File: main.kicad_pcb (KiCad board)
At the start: 2 copper layers, 82.8 x 33.2 mm, 34 parts, among them J1 USB_C_Receptacle_USB2.0_14P, SW1 SW_PUSH, SW2 SW_PUSH, SW3 SW_PUSH, SW4 SW_PUSH, SW5 SW_PUSH, U1 NCP1117-3.3_SOT223, U2 RP2040, U3 W25Q128JVS, Y1 ABM8-272-T3

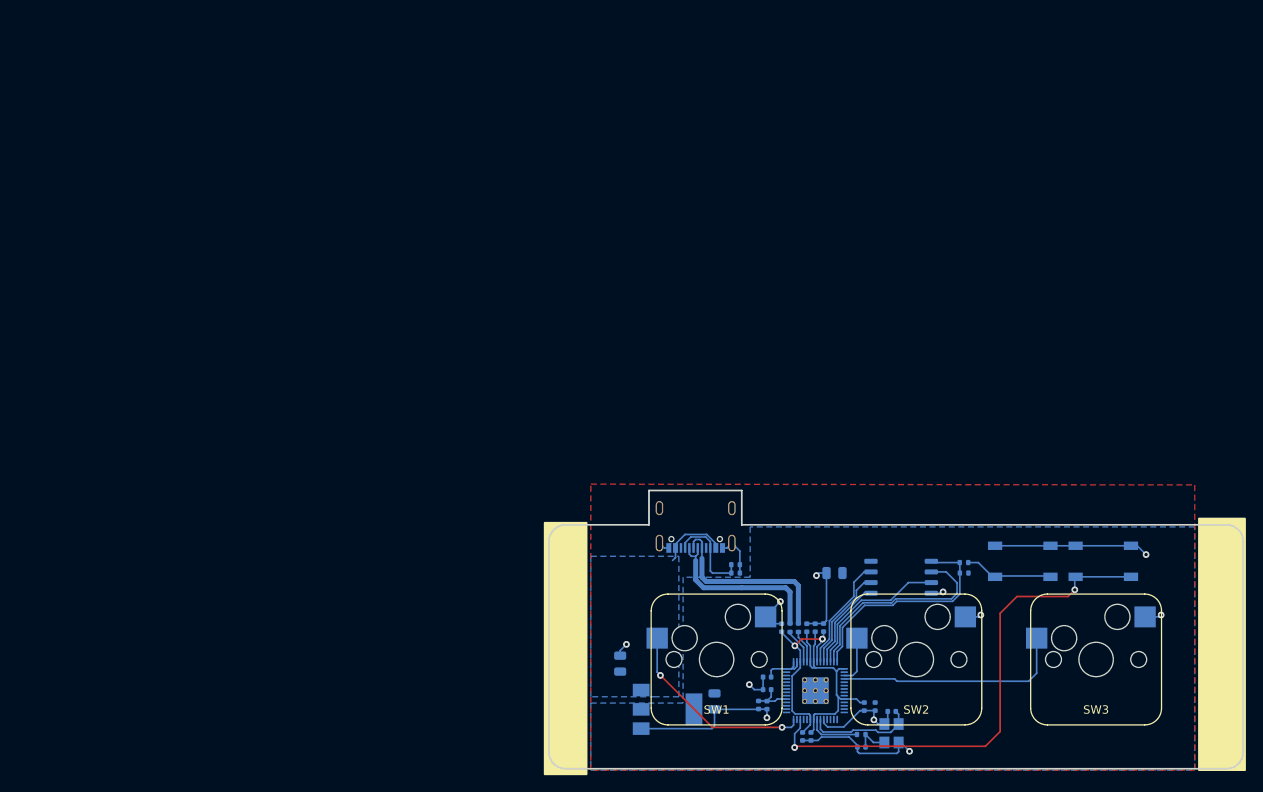
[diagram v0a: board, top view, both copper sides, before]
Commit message: :sparkles: (all) prepare fab
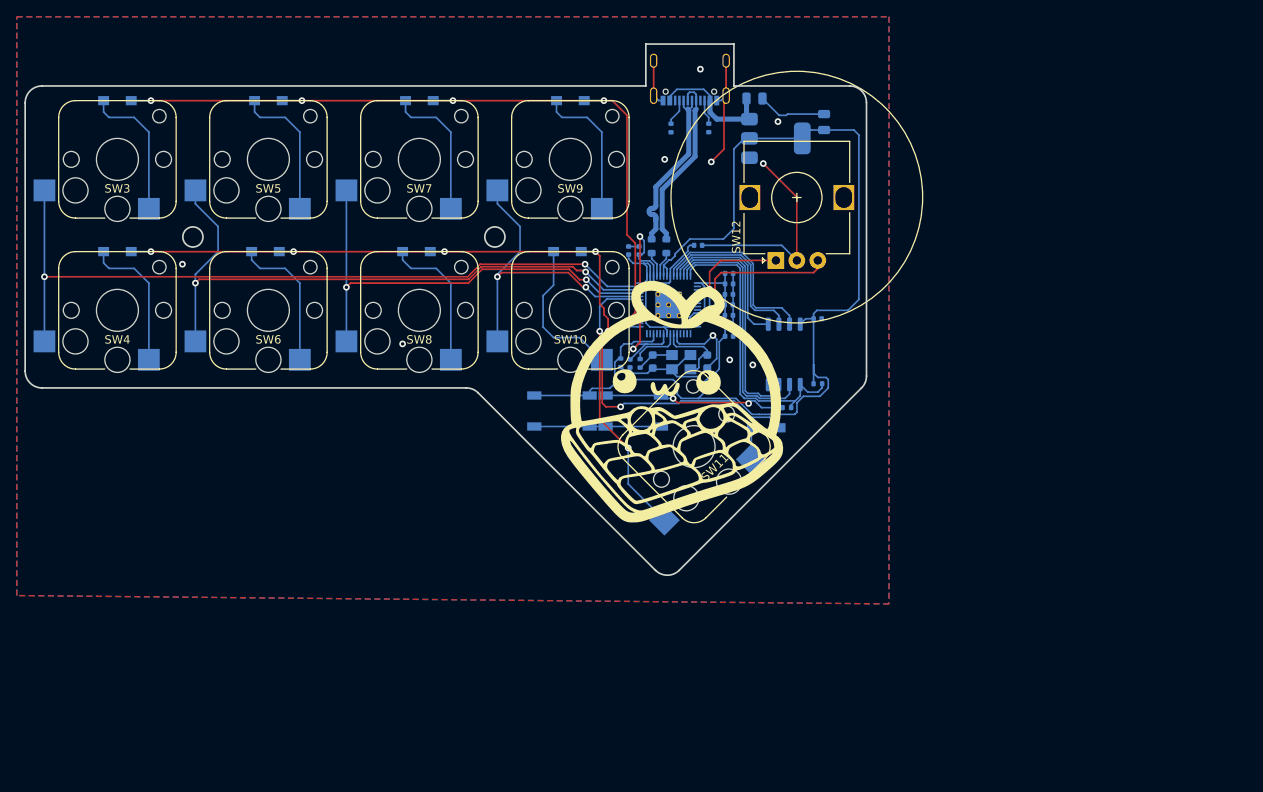
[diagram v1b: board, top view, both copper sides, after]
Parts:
- removed C17: 33p, Capacitor_SMD:C_0402_1005Metric
- added D1: D, kamo3_footprint:Diode_SOD123, B.Cu at (35.6, 24.2)
- added D2: D, kamo3_footprint:Diode_SOD123, B.Cu at (35.6, 42.2)
- added D3: D, kamo3_footprint:Diode_SOD123, B.Cu at (53.6, 24.2)
- added D4: D, kamo3_footprint:Diode_SOD123, B.Cu at (53.2, 42.2)
- added D5: D, kamo3_footprint:Diode_SOD123, B.Cu at (71.6, 24.2)
- added D6: D, kamo3_footprint:Diode_SOD123, B.Cu at (71.2, 42.2)
- added D7: D, kamo3_footprint:Diode_SOD123, B.Cu at (89.6, 24.2)
- added D8: D, kamo3_footprint:Diode_SOD123, B.Cu at (89.2, 42.2)
- added D9: D, kamo3_footprint:Diode_SOD123, B.Cu at (112.9, 63.2)
- added G***: LOGO, kamo3_footprint:logo, F.Cu at (102.1, 59.9)
- added R8: 1k, Resistor_SMD:R_0402_1005Metric, B.Cu at (97.9, 55.5)
- added SW10: SW_PUSH, kamo3_footprint:SW_ChocV1_Hotswap_1.0u, F.Cu at (89.6, 49.2)
- added SW11: SW_PUSH, kamo3_footprint:SW_ChocV1_Hotswap_1.50u, F.Cu at (104.3, 65.4)
- added SW12: RotaryEncoder, Rotary_Encoder:RotaryEncoder_Alps_EC12E_Vertical_H20mm, F.Cu at (114.1, 43.2)
- added SW6: SW_PUSH, kamo3_footprint:SW_ChocV1_Hotswap_1.0u, F.Cu at (53.6, 49.2)
- added SW7: SW_PUSH, kamo3_footprint:SW_ChocV1_Hotswap_1.0u, F.Cu at (71.6, 31.2)
- added SW8: SW_PUSH, kamo3_footprint:SW_ChocV1_Hotswap_1.0u, F.Cu at (71.6, 49.2)
- added SW9: SW_PUSH, kamo3_footprint:SW_ChocV1_Hotswap_1.0u, F.Cu at (89.6, 31.2)
- C10, C11: value 10u -> 100n; footprint Capacitor_SMD:C_0805_2012Metric -> Capacitor_SMD:C_0402_1005Metric
- C12, C13: value 1u -> 100n
- C15: value 10u -> 30p; footprint Capacitor_SMD:C_0805_2012Metric -> Capacitor_SMD:C_0603_1608Metric
- C16: value 33p -> 30p; footprint Capacitor_SMD:C_0402_1005Metric -> Capacitor_SMD:C_0603_1608Metric
- C3, C7: value 100n -> 1u
- C4, C5: value 100n -> 10u; footprint Capacitor_SMD:C_0402_1005Metric -> Capacitor_SMD:C_0805_2012Metric
- R1: value 5.1k -> 10k
- R3: value 27 -> 5.1k
- R4: value 27 -> 1k
- R5: value DNF -> 27; footprint Resistor_SMD:R_0402_1005Metric -> Resistor_SMD:R_0603_1608Metric
- R6: value 1k -> 27; footprint Resistor_SMD:R_0402_1005Metric -> Resistor_SMD:R_0603_1608Metric
- R7: value 1k -> DNF
- SW1, SW2: footprint kamo3_footprint:SW_CherryMX_Hotswap_1.25u -> kamo3_footprint:Tact_Switch_5.1_5.1mm_SMD; moved to B.Cu
- SW3: footprint kamo3_footprint:SW_CherryMX_Hotswap_1.00u -> kamo3_footprint:SW_ChocV1_Hotswap_1.0u
- SW4, SW5: footprint kamo3_footprint:Tact_Switch_5.1_5.1mm_SMD -> kamo3_footprint:SW_ChocV1_Hotswap_1.0u; moved to F.Cu
- moved SW3 131.0 mm to (35.6, 31.2)
- moved SW4 121.3 mm to (35.6, 49.2), turned to 0 degrees
- moved SW5 101.9 mm to (53.6, 31.2), turned to 0 degrees
- moved C5 70.0 mm to (119.8, 26.7), turned to 90 degrees
- moved U1 69.3 mm to (114.1, 28.7)
- moved C4 63.5 mm to (111.5, 23.9), turned to 0 degrees
- moved R3 61.5 mm to (101.6, 27.4), turned to 90 degrees
- moved C3 60.6 mm to (97.8, 42.0), turned to 90 degrees
- moved C7 56.4 mm to (96.5, 42.0), turned to 90 degrees
- moved C9 53.6 mm to (108.5, 47.3), turned to 0 degrees
- moved J1 53.3 mm to (103.8, 21.7)
- moved R2 53.2 mm to (106.1, 27.4), turned to 90 degrees
- moved R6 53.0 mm to (99.3, 41.5), turned to -90 degrees
- moved R5 52.7 mm to (101.0, 41.5), turned to -90 degrees
- moved C6 51.7 mm to (108.5, 44.8), turned to 0 degrees
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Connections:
- C10 pad 1: VBUS -> +3V3
- C12 pad 1: +1V1 -> +3V3
- C15 pad 1: +3V3 -> GND
- C15 pad 2: GND -> /XIN
- C16 pad 1: /XIN -> GND
- C16 pad 2: GND -> Net-(C16-Pad2)
- C3 pad 1: +3V3 -> +1V1
- C4 pad 1: +3V3 -> VBUS
- J1 pad B5: Net-(J1-CC1) -> Net-(J1-CC2)
- R1 pad 1: Net-(J1-CC1) -> +3V3
- R1 pad 2: GND -> Net-(U2-RUN)
- R2 pad 1: Net-(J1-CC1) -> GND
- R2 pad 2: GND -> Net-(J1-CC2)
- R3 pad 1: /USB_D+ -> GND
- R3 pad 2: Net-(U2-USB_DP) -> Net-(J1-CC1)
- R4 pad 1: /USB_D- -> /QSPI_SS
- R4 pad 2: Net-(U2-USB_DM) -> Net-(R4-Pad2)
- R5 pad 1: +3V3 -> /USB_D+
- R5 pad 2: /QSPI_SS -> Net-(U2-USB_DP)
- R6 pad 1: /QSPI_SS -> /USB_D-
- R6 pad 2: /~{USB_BOOT} -> Net-(U2-USB_DM)
- R7 pad 1: /XOUT -> +3V3
- R7 pad 2: Net-(C17-Pad1) -> /QSPI_SS
- SW1 pad 1: Net-(U2-GPIO17) -> GND
- SW2 pad 1: Net-(U2-GPIO1) -> GND
- SW3 pad 1: Net-(U2-GPIO2) -> /col0
- SW3 pad 2: GND -> Net-(D1-A)
- SW4 pad 1: GND -> /col0
- SW4 pad 2: GND -> Net-(D2-A)
- SW5 pad 1: GND -> /col1
- SW5 pad 2: GND -> Net-(D3-A)
- U2 pad 11: unconnected-(U2-GPIO8-Pad11) -> /enc_a
- U2 pad 12: unconnected-(U2-GPIO9-Pad12) -> /enc_b
- U2 pad 28: Net-(U2-GPIO17) -> unconnected-(U2-GPIO17-Pad28)
- U2 pad 29: unconnected-(U2-GPIO18-Pad29) -> /row1
- U2 pad 3: Net-(U2-GPIO1) -> unconnected-(U2-GPIO1-Pad3)
- U2 pad 30: unconnected-(U2-GPIO19-Pad30) -> /row0
- U2 pad 37: unconnected-(U2-GPIO25-Pad37) -> /col4
- U2 pad 38: unconnected-(U2-GPIO26_ADC0-Pad38) -> /col3
- U2 pad 39: unconnected-(U2-GPIO27_ADC1-Pad39) -> /col2
- U2 pad 4: Net-(U2-GPIO2) -> unconnected-(U2-GPIO2-Pad4)
- U2 pad 40: unconnected-(U2-GPIO28_ADC2-Pad40) -> /col1
- U2 pad 41: unconnected-(U2-GPIO29_ADC3-Pad41) -> /col0
- Y1 pad 3: Net-(C17-Pad1) -> Net-(C16-Pad2)
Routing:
- net +3V3: track 37.5 -> 155.2 mm
- net /row1: track 0.00 -> 106.4 mm, vias 0 -> 6
- net /row0: track 0.00 -> 93.9 mm, vias 0 -> 5
- net /col0: track 0.00 -> 90.7 mm, vias 0 -> 2
- net /col1: track 0.00 -> 75.2 mm, vias 0 -> 2
- net /col2: track 0.00 -> 55.1 mm, vias 0 -> 2
- net Net-(U2-RUN): track 61.1 -> 20.3 mm, vias 2 -> 0
- net /col3: track 0.00 -> 38.6 mm, vias 0 -> 2
- net /col4: track 0.00 -> 33.9 mm, vias 0 -> 2
- net Net-(U2-GPIO2): track 27.6 -> 0.00 mm
- net Net-(U2-GPIO17): track 23.8 -> 0.00 mm, vias 2 -> 0
- net Net-(R4-Pad2): track 0.00 -> 21.5 mm, vias 0 -> 2
- net /enc_b: track 0.00 -> 19.8 mm, vias 0 -> 1
- net Net-(D8-A): track 0.00 -> 18.1 mm
- net Net-(D6-A): track 0.00 -> 17.0 mm
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- added copper zone on B.Cu, net GND
- removed copper zone on B.Cu, net +3V3
- removed copper zone on B.Cu, net VBUS
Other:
- board size 82.8 x 33.2 mm -> 100.3 x 63.3 mm
